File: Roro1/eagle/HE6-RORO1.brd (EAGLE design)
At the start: 50.8 x 27.9 mm, 23 parts, among them U3 ESP32-WROOM-32(8MB)

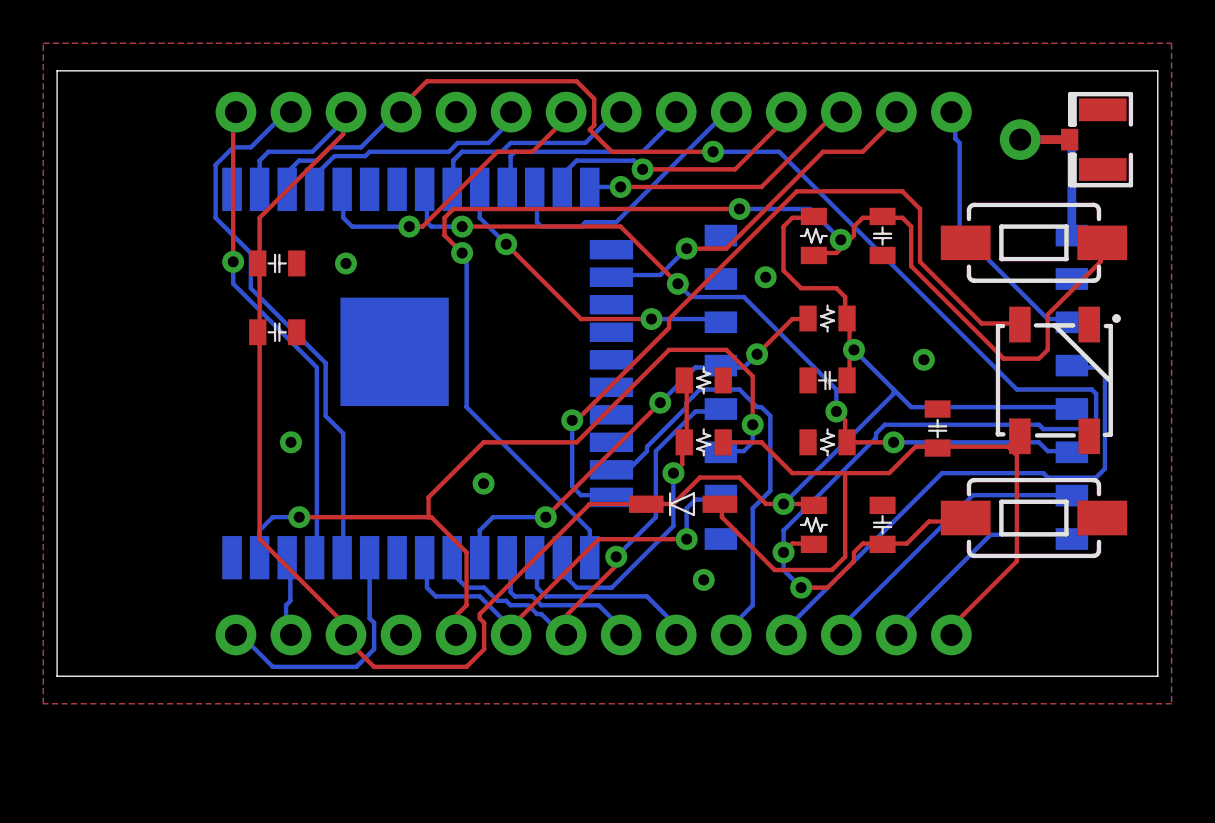
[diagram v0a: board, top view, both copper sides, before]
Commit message: .
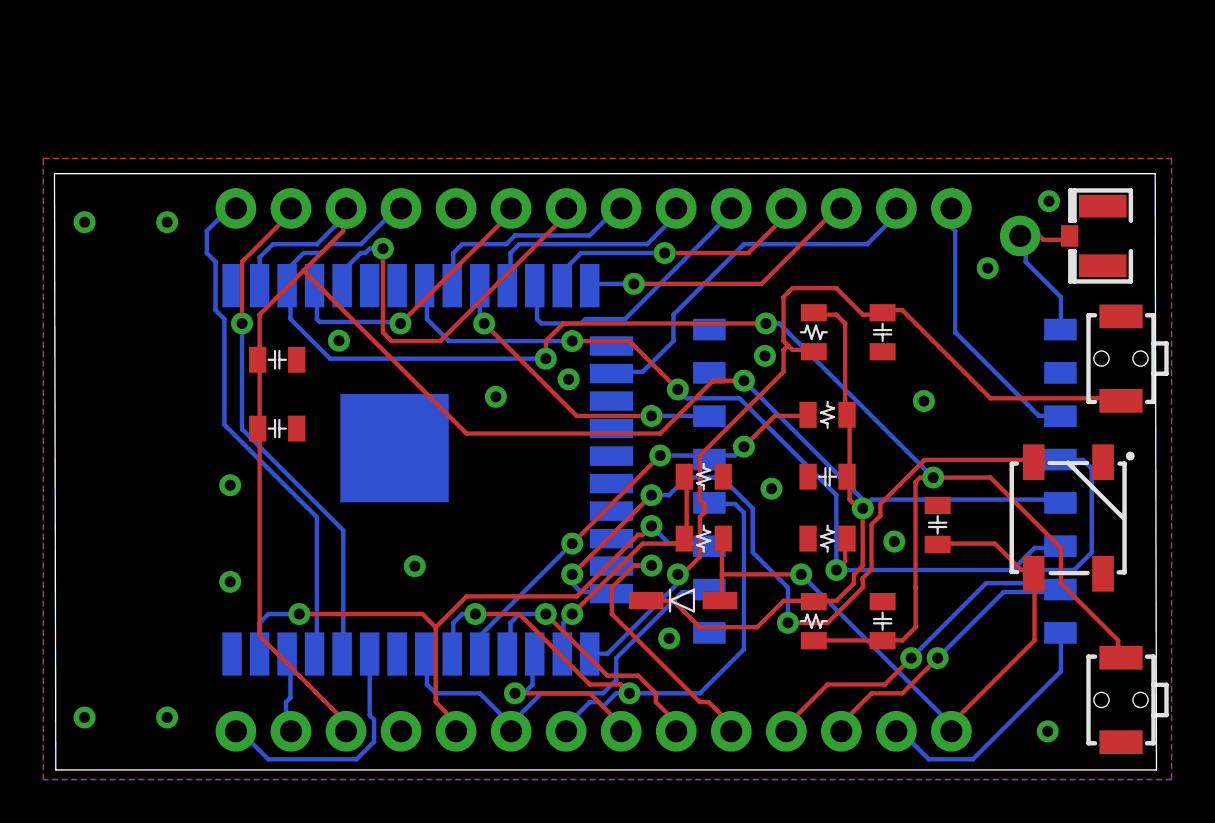
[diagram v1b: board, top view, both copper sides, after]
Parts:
- PGM, RST: value MOMENTARY-SWITCH-SPST-SMD-6.0X3.5MM -> MOMENTARY-SWITCH-SPST-SMD-RIGHT-ANGLE; device SparkFun-Switches:TACTILE_SWITCH_SMD_6.0X3.5MM -> SparkFun-Switches:TACTILE_SWITCH_SMD_RIGHT_ANGLE
- moved RST 9.31 mm to (49.1, 3.35), turned to 90 degrees
- moved PGM 6.68 mm to (49.1, 19.1), turned to 90 degrees
- moved NEO 6.38 mm to (46.7, 11.7)
- moved ANT 4.45 mm to (48.3, 24.8)
- moved C1 4.45 mm to (40.6, 11.4)
- moved C10 4.45 mm to (10.2, 19.1)
- moved C12 4.45 mm to (38.1, 20.3)
- moved C2 4.45 mm to (35.6, 13.7)
- moved C9 4.45 mm to (10.2, 15.9)
- moved D2 4.45 mm to (28.9, 7.94)
- moved J1 4.45 mm to (44.5, 24.8)
- moved J4 4.45 mm to (41.3, 26.0)
- moved R1 4.45 mm to (29.8, 13.7)
- moved R4 4.45 mm to (29.8, 10.8)
- moved R5 4.45 mm to (34.9, 20.3)
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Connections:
- net RXD2: now also U3.27; no longer U3.28
- net TXD2: now also U3.28; no longer U3.27
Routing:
- net PGM: track 59.5 -> 40.5 mm, vias 3 -> 1
- net +3V3: track 91.7 -> 101.3 mm
- net RST: track 79.1 -> 69.6 mm
- net MOSI: track 39.6 -> 30.2 mm
- net SCK: track 21.2 -> 29.6 mm, vias 1 -> 2
- net IO15: track 20.5 -> 13.4 mm, vias 0 -> 1
- net VBAT: track 36.6 -> 30.8 mm, vias 0 -> 1
- net VN: track 14.2 -> 18.2 mm
- net TXD2: track 8.99 -> 12.1 mm, vias 0 -> 1
- net BATV: track 14.5 -> 11.6 mm
- net RFM_DIO0: track 36.9 -> 39.8 mm, vias 4 -> 3
- net VP: track 11.1 -> 13.2 mm, vias 0 -> 1
- net N$1: track 9.10 -> 7.53 mm
- net RXD0: track 25.1 -> 23.7 mm, vias 0 -> 1
- net DIO2: track 10.4 -> 11.7 mm
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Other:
- board size 50.8 x 27.9 mm -> 50.9 x 27.5 mm
